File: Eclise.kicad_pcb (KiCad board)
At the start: 2 copper layers, 80.2 x 104.6 mm, 19 parts, among them J1 Power Supply, J10 Sensor_Power, J11 Sensor_GND, J12 Sensor_Power, J13 Sensor_GND, J14 D12-D13, J2 AMS_In, J3 AMS_Out, J4 Prog_Pins, J5 Prog_Power, J6 A0-A3, J7 A4-A7, J8 D2-D5, J9 D6-D9, U1 ESP-01S

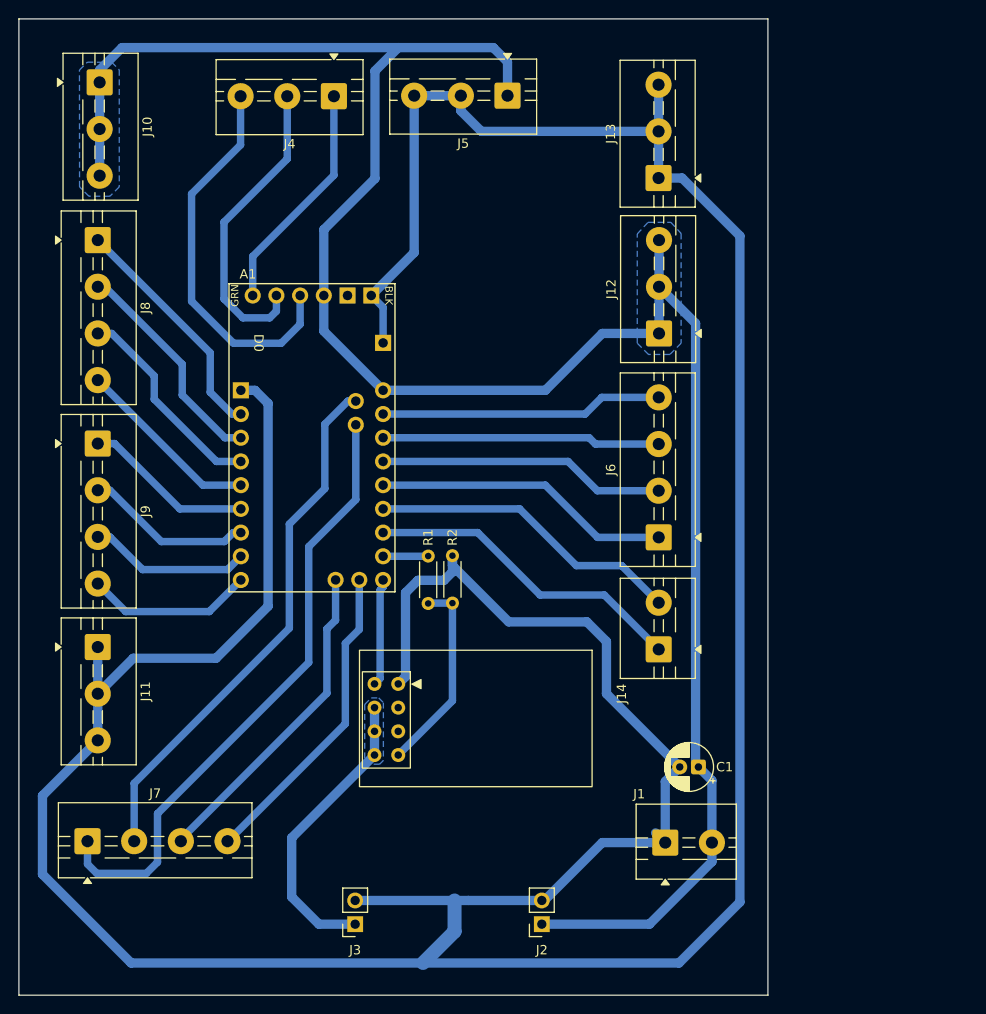
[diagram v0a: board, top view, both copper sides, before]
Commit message: Rearrangement of PCB
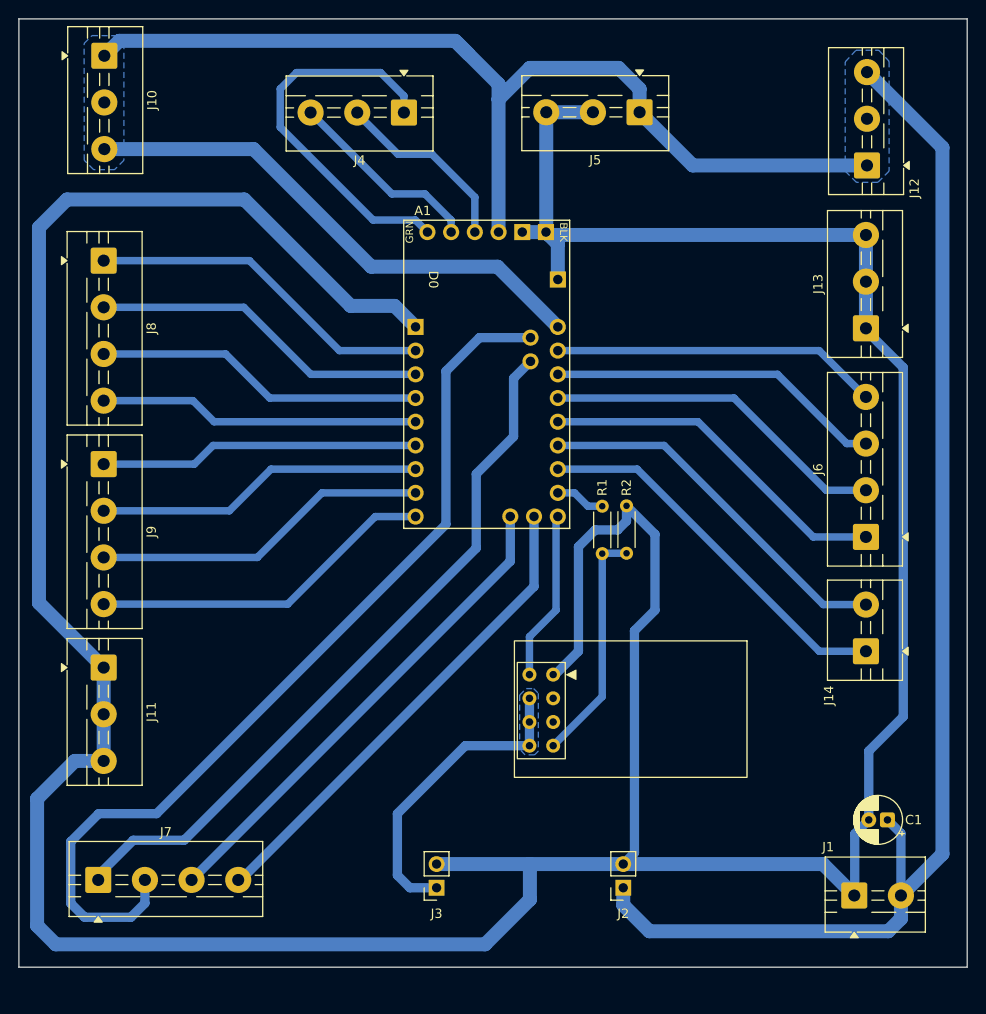
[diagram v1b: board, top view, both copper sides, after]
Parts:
- moved J12 28.6 mm to (179.1, 65.0)
- moved J13 27.4 mm to (179.0, 82.4)
- moved J14 22.2 mm to (179.0, 117.0)
- moved J6 22.2 mm to (179.0, 104.8)
- moved C1 21.0 mm to (181.3, 135.1)
- moved J1 21.0 mm to (177.8, 143.2)
- moved A1 19.9 mm to (138.4, 87.3)
- moved R1 19.4 mm to (150.8, 101.5)
- moved R2 19.4 mm to (153.3, 101.4)
- moved U1 16.6 mm to (145.5, 119.5)
- moved J5 14.3 mm to (154.8, 59.2)
- moved J2 9.56 mm to (153.0, 142.3)
- moved J3 9.56 mm to (133.0, 142.3)
- moved J4 7.70 mm to (129.5, 59.3)
- moved J7 4.31 mm to (96.8, 141.5)
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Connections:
- A1 pad GND4: (no net) -> GND
- J4 pad 2: /TXO -> /RXI
- J4 pad 3: /RXI -> /TXO
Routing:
- net 5V: track 230.0 -> 303.4 mm
- net Net-(A1-A5/SCL): track 57.5 -> 99.5 mm
- net GND: track 415.4 -> 454.2 mm
- net /RXI: track 41.6 -> 20.2 mm
- net Net-(J9-Pin_4): track 18.0 -> 37.3 mm
- net Net-(J9-Pin_3): track 17.4 -> 36.3 mm
- net Net-(J7-Pin_4): track 33.9 -> 52.2 mm
- net Net-(J7-Pin_3): track 34.9 -> 53.1 mm
- net Net-(J9-Pin_2): track 18.0 -> 35.3 mm
- net /DTR: track 25.0 -> 41.3 mm
- net Net-(J9-Pin_1): track 18.2 -> 34.2 mm
- net Net-(J8-Pin_4): track 20.0 -> 34.4 mm
- net Net-(J8-Pin_3): track 22.5 -> 35.4 mm
- net Net-(A1-D3_INT1): track 24.0 -> 36.4 mm
- net Net-(A1-D2_INT0): track 25.5 -> 37.4 mm
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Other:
- board size 80.2 x 104.6 mm -> 101.6 x 101.6 mm
